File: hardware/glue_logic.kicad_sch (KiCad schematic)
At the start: 30 parts, among them U13 74AHC74, U14 74AHC125, U15 DS1035-10, U16 74AHC00, U17 74AHC02, U18 74AHC32, U19 74AC10, U20 74ACT245, U21 74AC563

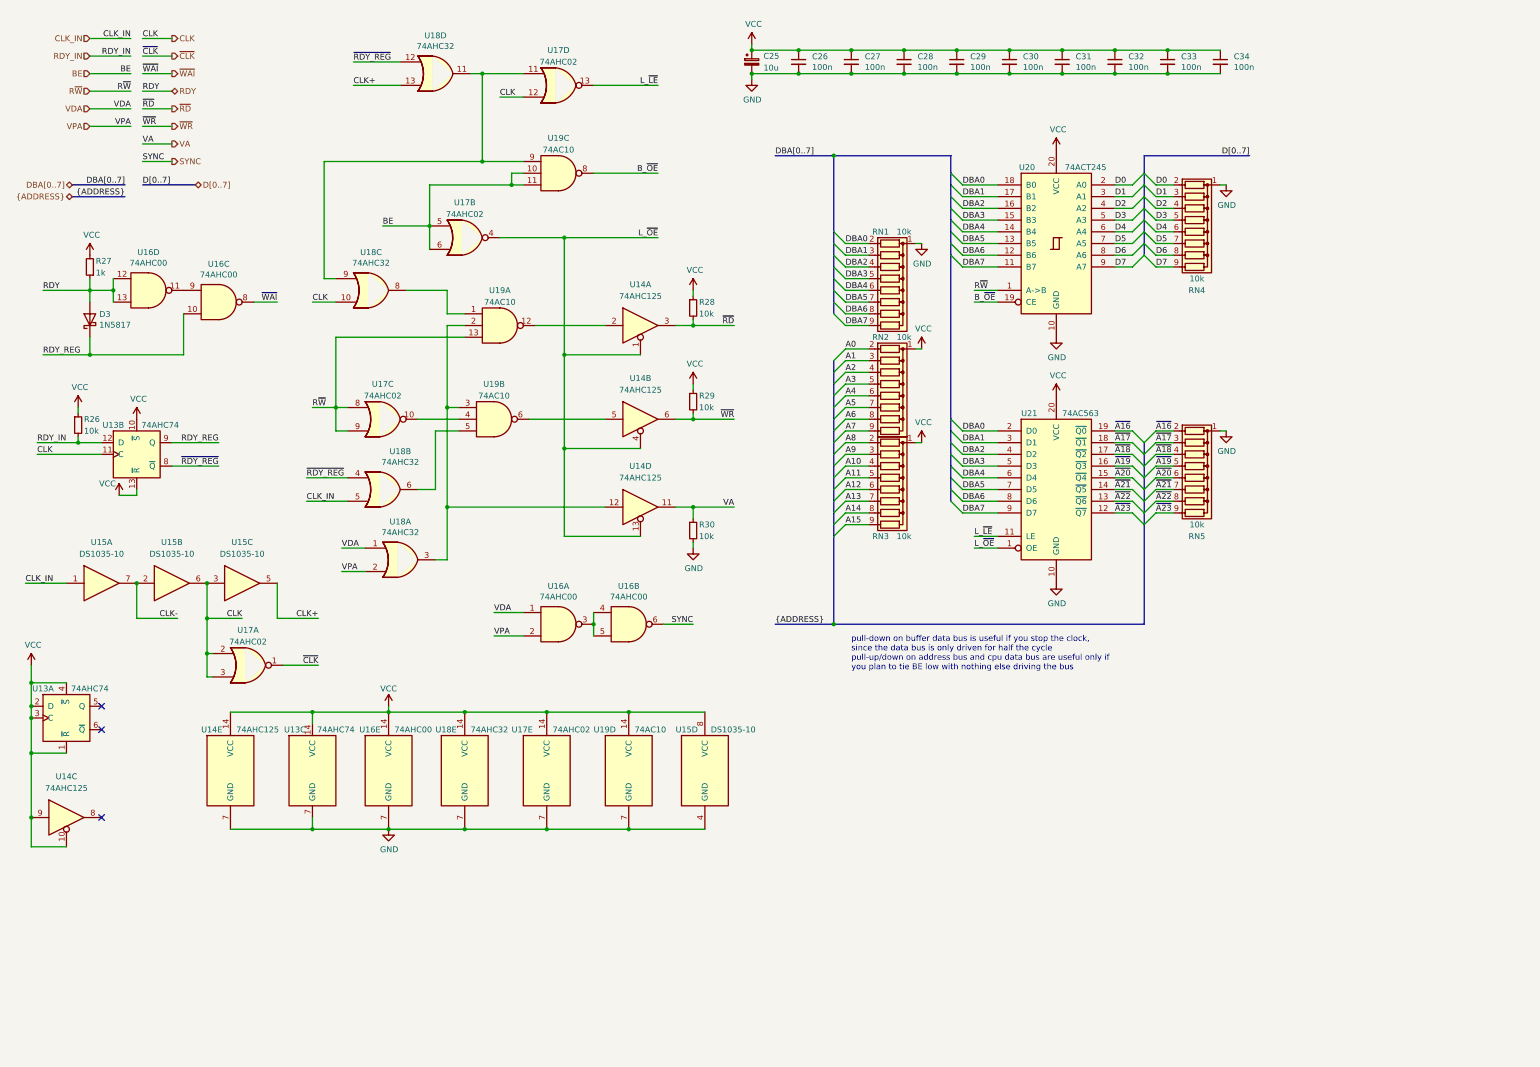
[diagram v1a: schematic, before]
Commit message: Update for episode 23
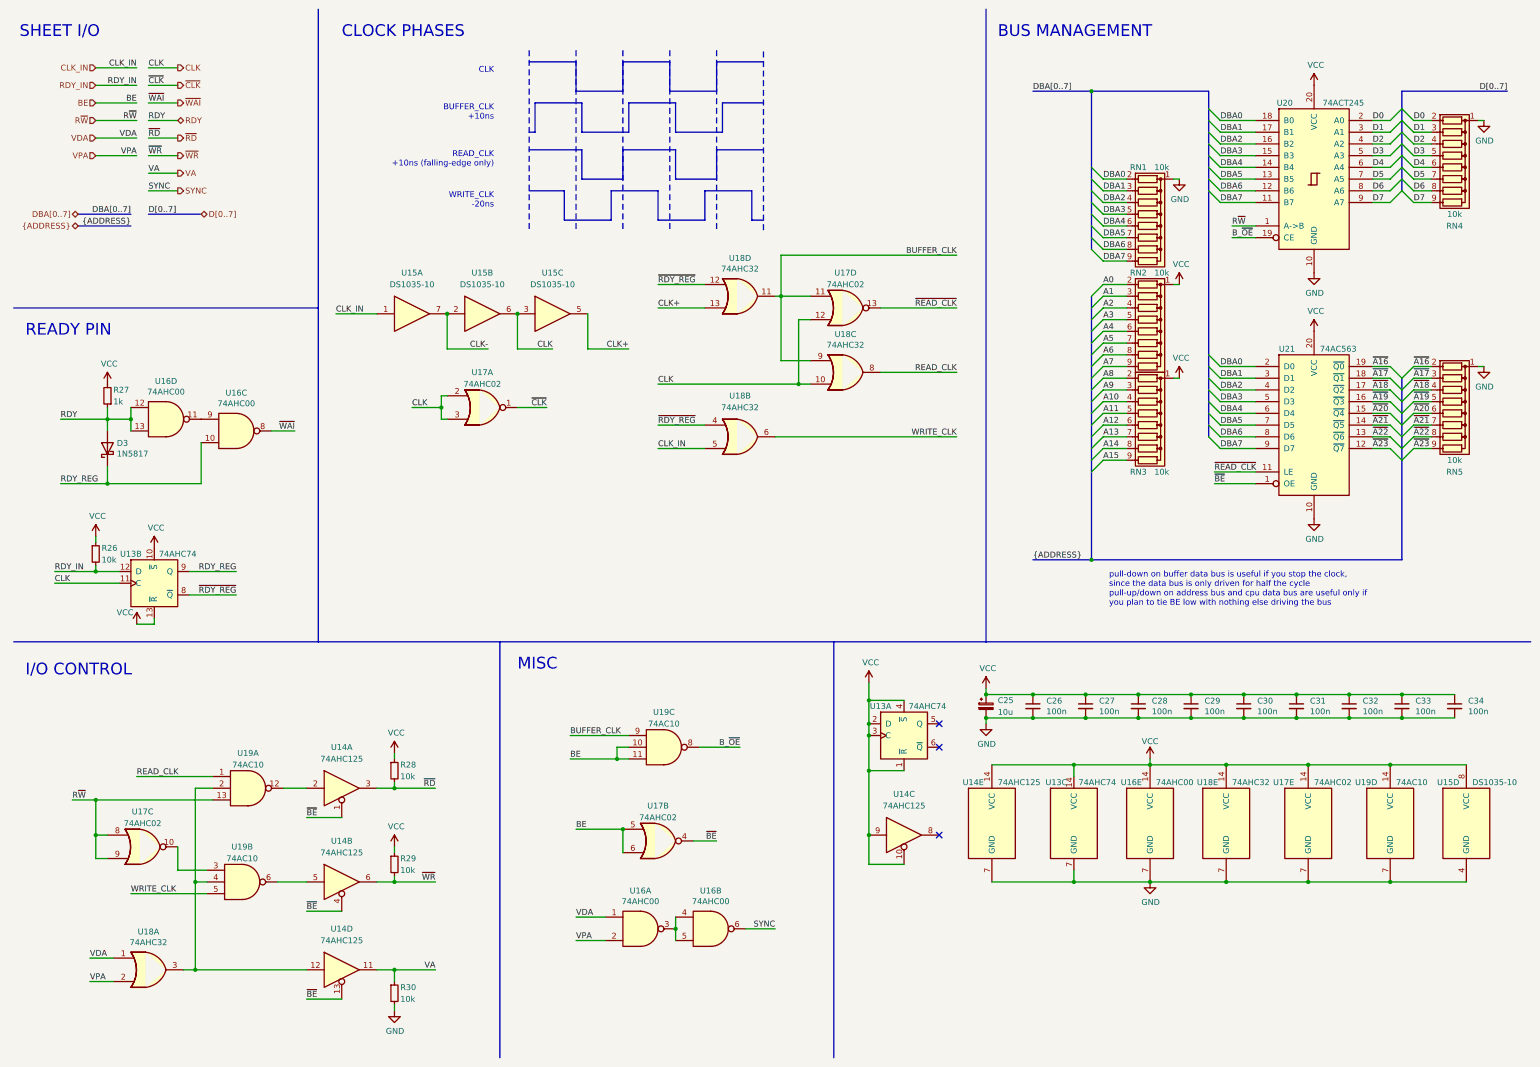
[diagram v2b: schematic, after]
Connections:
- net BUFFER_CLK: now reaches U17.11, U18.11, U18.9, U19.9
- net at U17.10: now also U19.3; no longer U19.4
- net WRITE_CLK: now reaches U18.6, U19.5
- net READ_CLK: now reaches U18.8, U19.1
- net at U14.12, U18.3, U19.2: now also U19.4; no longer U19.3
- net L_~{LE} renamed ~{READ_CLK}
- net L_~{OE} renamed ~{BE}
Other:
- note added: "BUFFER_CLK +10ns"
- note added: "BUS MANAGEMENT"
- note added: "CLK"
- note added: "CLOCK PHASES"
- note added: "I/O CONTROL"
- note added: "MISC"
- note added: "READY PIN"
- note added: "READ_CLK +10ns (falling-edge only)"
- note added: "SHEET I/O"
- note added: "WRITE_CLK -20ns"
- moved on the sheet: C25, C26, C27, C28, C29, C30, C31, C32, C33, C34, D3, R26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
